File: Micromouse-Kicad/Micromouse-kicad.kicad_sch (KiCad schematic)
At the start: 97 parts, among them J1 SWD, J2 USB_B_Micro, J3 UARTBTH, J4 Batería, J5 VL6180x, J6 MotorEncodL, J7 MotorEncodR, Q1 BS170, Q2 BS170, Q3 BS170, Q4 BS170, SW1 RST, SW2 BootSwitch, SW3 PowerSwitch, SW4 BTN, SW5 BTN, U1 STM32F405RGT6, U10 TCRT5000, U2 AMS1117-5.0, U3 AMS1117-3.3, U4 SRV05-4, U5 MPU-6500, U6 DRV8833PWPR, U7 TCRT5000, U8 TCRT5000, U9 TCRT5000, Y1 8MHz

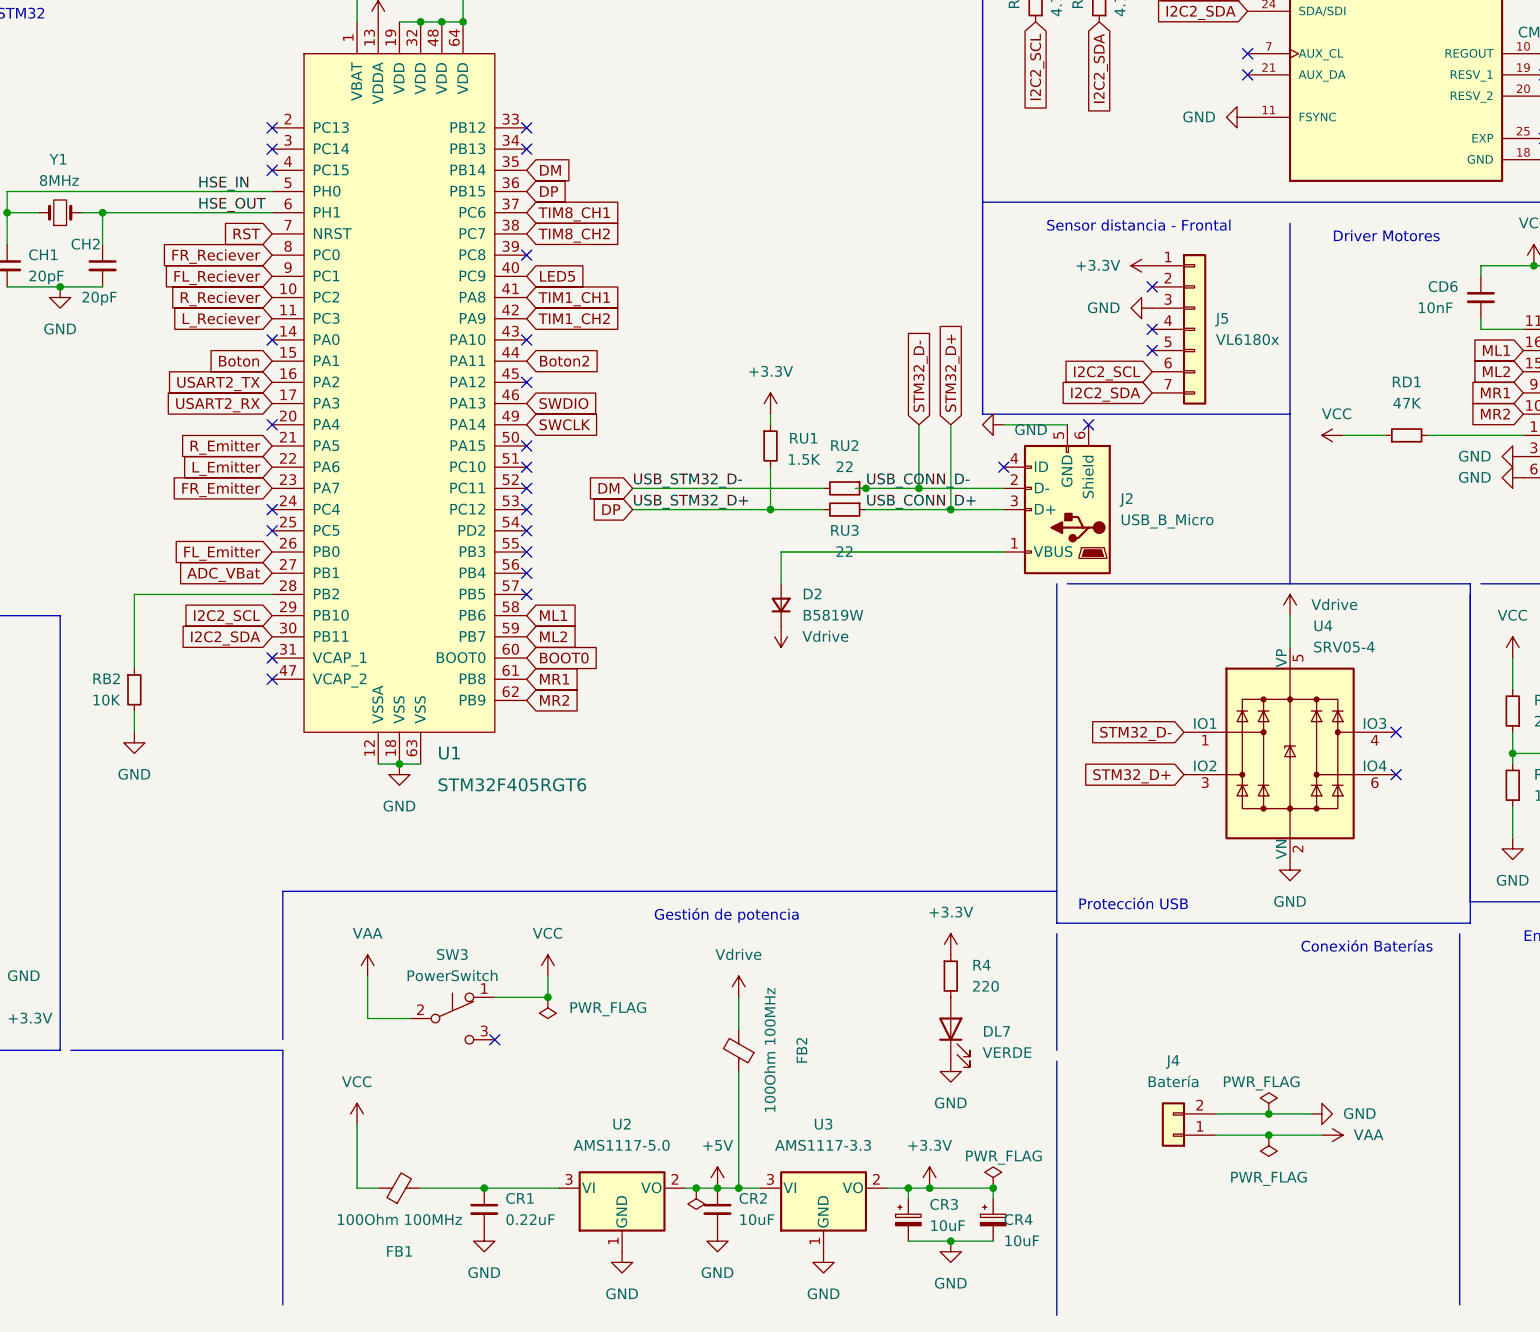
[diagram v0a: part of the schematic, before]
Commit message: Fabricado!
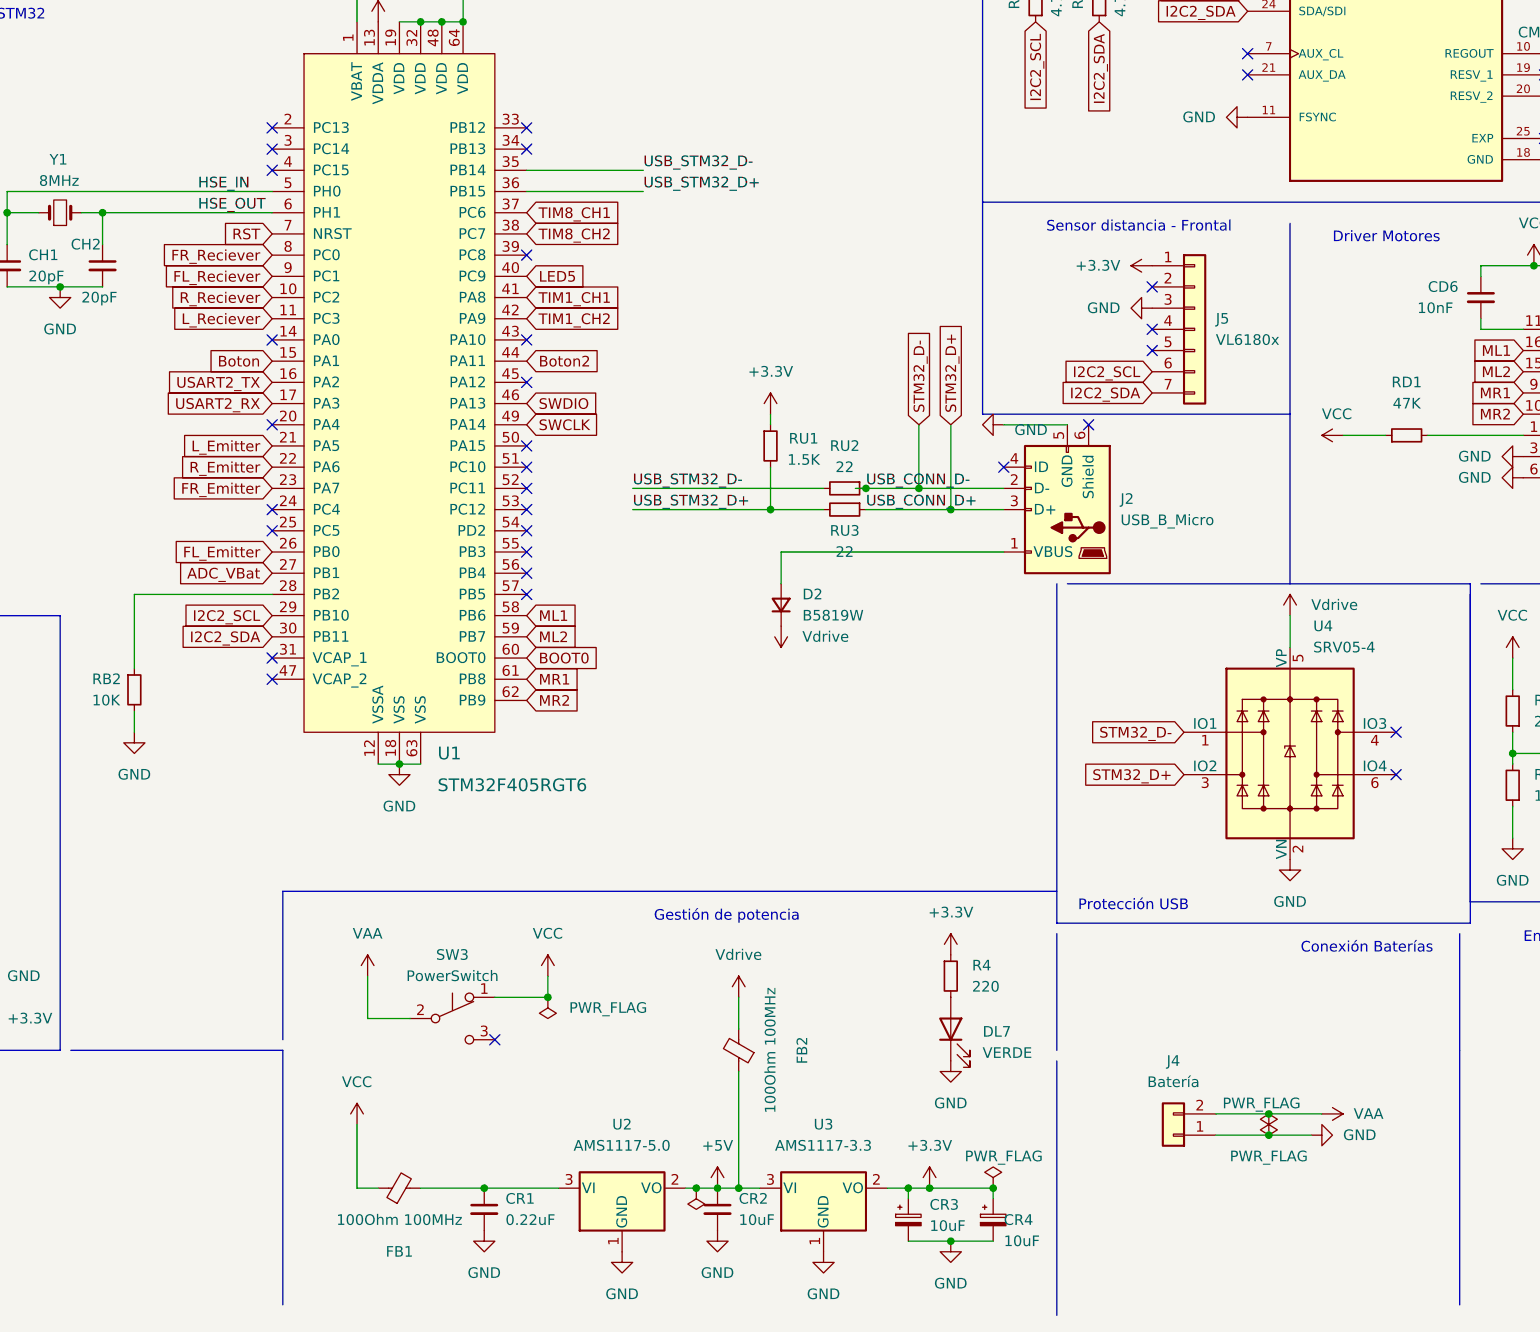
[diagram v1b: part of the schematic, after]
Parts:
- J6, J7: footprint Connector_JST:JST_SHL_SM06B-SHLS-TF_1x06-1MP_P1.00mm_Horizontal -> Connector_JST:JST_SH_BM06B-SRSS-TB_1x06-1MP_P1.00mm_Vertical
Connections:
- net GND: now also J4.1 (Pin_1); no longer J4.2 (Pin_2)
- net L_Emitter: now also U1.21 (PA5); no longer U1.22 (PA6)
- net R_Emitter: now also U1.22 (PA6); no longer U1.21 (PA5)
- net VAA: now also J4.2 (Pin_2); no longer J4.1 (Pin_1)
- net DM renamed USB_STM32_D-
- net DP renamed USB_STM32_D+
